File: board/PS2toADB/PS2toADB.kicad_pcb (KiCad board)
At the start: 2 copper layers, 36.9 x 33.6 mm, 7 parts, among them U1 PIC12F1840

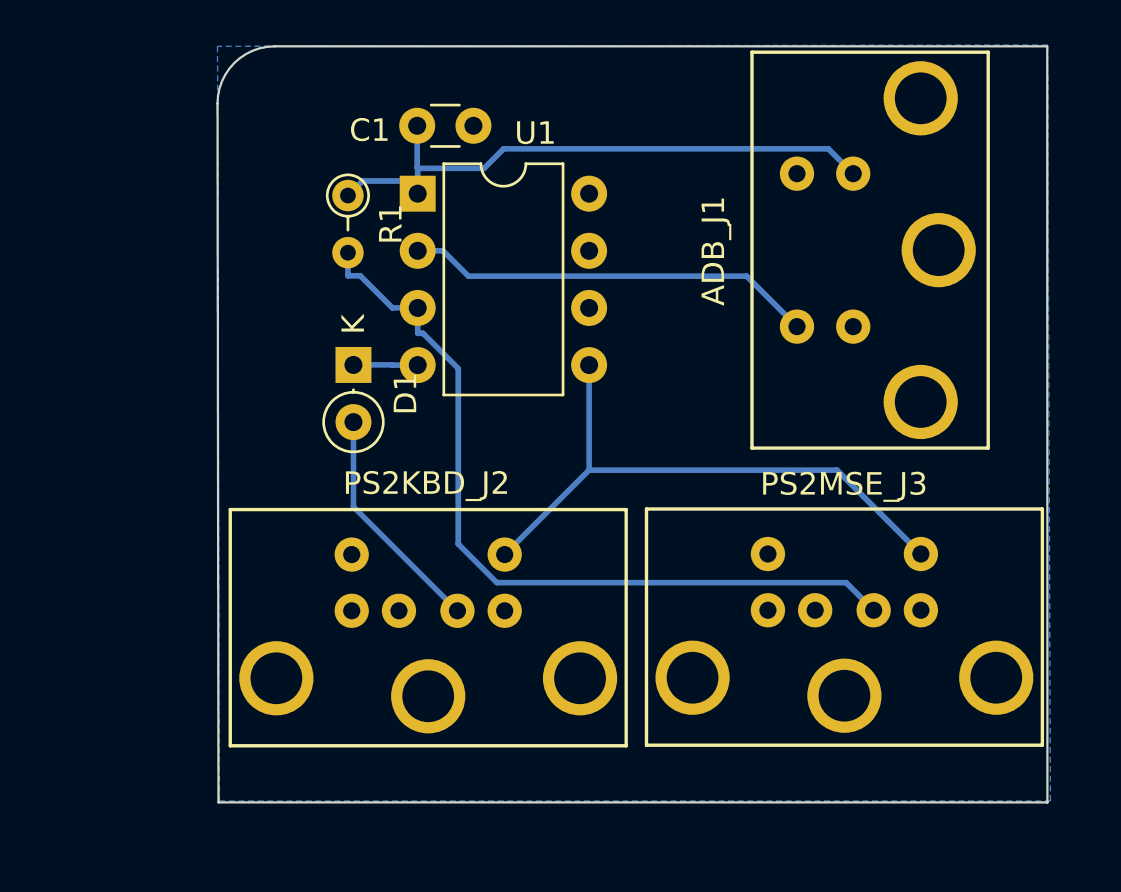
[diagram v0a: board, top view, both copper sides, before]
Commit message: Updated schematic. Added power button and renders
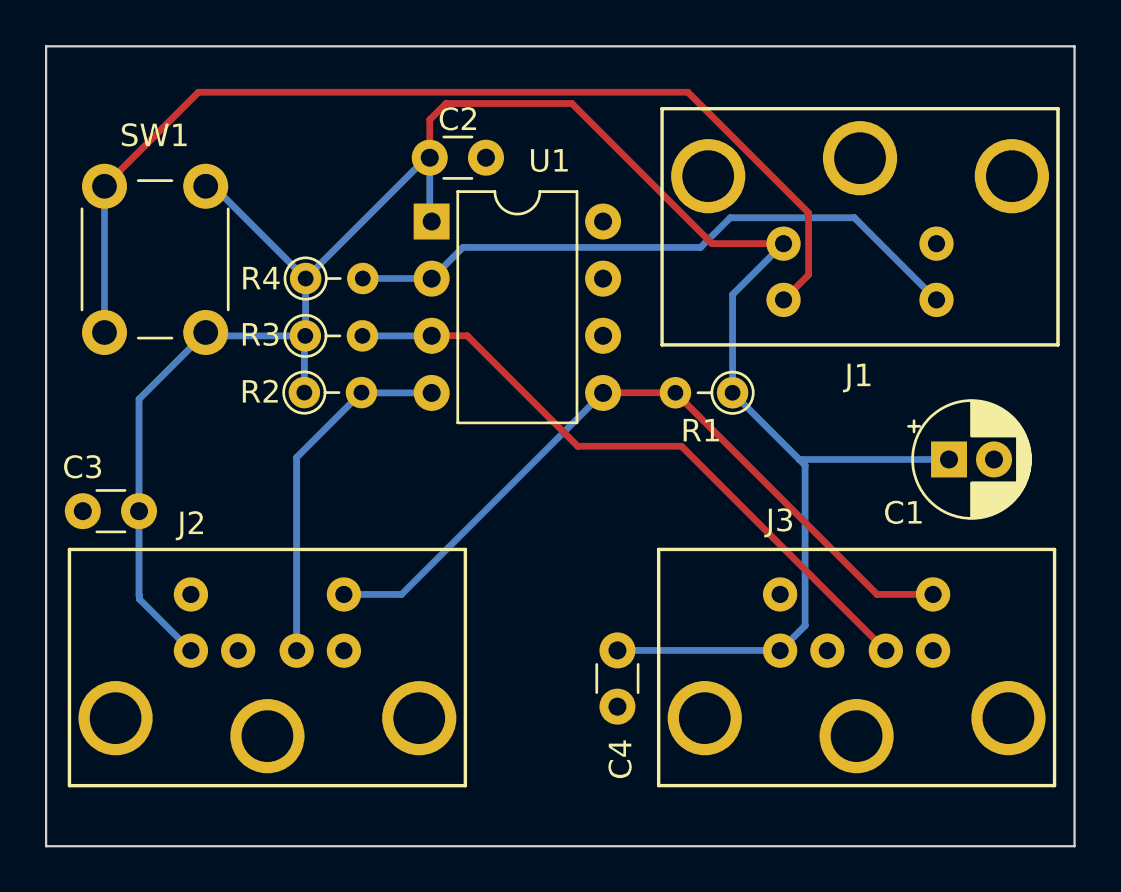
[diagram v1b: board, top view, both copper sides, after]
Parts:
- removed D1: 1N4148, Diode_THT:D_DO-35_SOD27_P2.54mm_Vertical_KathodeUp
- added C1: 10 uF, Capacitor_THT:CP_Radial_D5.0mm_P2.00mm, F.Cu at (174.8, 38.7)
- added C3: 470 nF, Capacitor_THT:C_Disc_D3.0mm_W1.6mm_P2.50mm, F.Cu at (138.8, 41.0)
- added C4: 470 nF, Capacitor_THT:C_Disc_D3.0mm_W1.6mm_P2.50mm, F.Cu at (160.0, 47.2)
- added R1: 5K, Resistor_THT:R_Axial_DIN0204_L3.6mm_D1.6mm_P2.54mm_Vertical, F.Cu at (165.1, 35.7)
- added R2: 5K, Resistor_THT:R_Axial_DIN0204_L3.6mm_D1.6mm_P2.54mm_Vertical, F.Cu at (146.1, 35.7)
- added R4: 10K, Resistor_THT:R_Axial_DIN0204_L3.6mm_D1.6mm_P2.54mm_Vertical, F.Cu at (146.2, 30.6)
- added SW1: PowerOn, Button_Switch_THT:SW_PUSH_6mm_H5mm, F.Cu at (141.7, 26.5)
- J1: renamed from ADB_J1; value Mini-DIN-4 -> ADB
- J2: renamed from PS2KBD_J2; value Mini-DIN-6 -> PS/2 Keyboard
- J3: renamed from PS2MSE_J3; value Mini-DIN-6 -> PS/2 Mouse
- R3: renamed from R1; value 100 -> 5K
- moved J1 12.0 mm to (170.8, 20.6), turned to 0 degrees
- moved J2 7.37 mm to (144.5, 55.7)
- moved R3 6.52 mm to (146.1, 33.2), turned to 0 degrees
- moved J3 1.88 mm to (170.7, 55.7)
- moved C2 1.53 mm to (151.7, 25.3)
- moved U1 1.38 mm to (151.8, 28.1)
- renumbered C1 to C2
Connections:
- net /PS2_MSE_DATA renamed /PS2_DTM
- J1 pad 2: unconnected-(ADB_J1-Pad2) -> /ADB_PWRON
- J2 pad 1: /PS2_KBD_DATA -> /PS2_DTK
- J2 pad 4: unconnected-(PS2KBD_J2-Pad4) -> VCC
- J3 pad 4: unconnected-(PS2MSE_J3-Pad4) -> VCC
- U1 pad 4: Net-(D1-K) -> /PS2_DTK
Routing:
- net VCC: track 26.6 -> 97.7 mm
- net /ADB_PWRON: track 0.00 -> 46.1 mm
- net /PS2_DTK: track 0.00 -> 15.8 mm
- net /PS2_KBD_DATA: track 10.3 -> 0.00 mm
- net /ADB_DATA: track 18.3 -> 28.1 mm
- net /PS2_CLK: track 26.3 -> 33.6 mm
- net /PS2_DTM: track 35.8 -> 29.1 mm
- net Net-(D1-K): track 2.86 -> 0.00 mm
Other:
- board size 36.9 x 33.6 mm -> 45.7 x 35.6 mm
